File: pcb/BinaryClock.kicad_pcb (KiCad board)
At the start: 2 copper layers, 26.4 x 41.7 mm, 17 parts, among them CON1 AVR-ISP-6, IC1 ATMEGA328P-A, U1 MC33269, U3 clock_header, U4 clock_header, U5 clock_header, Y1 16MHz

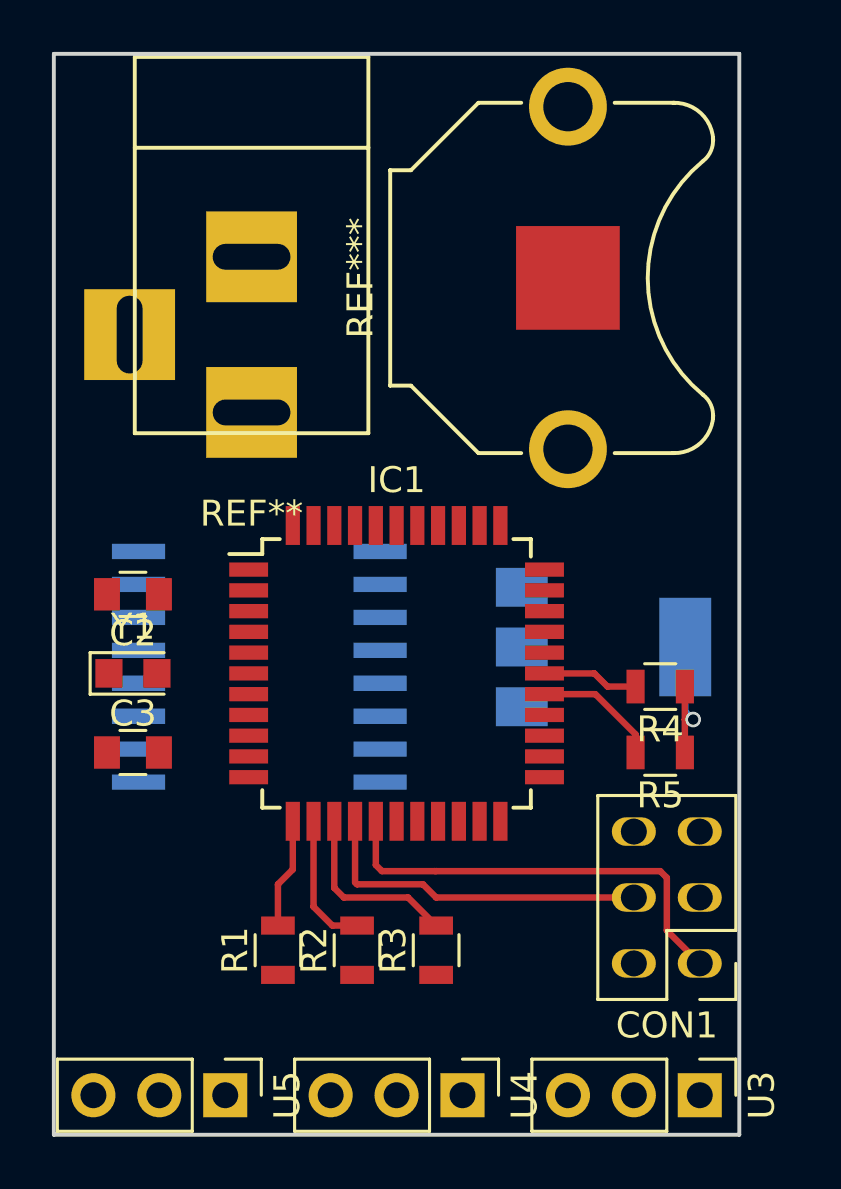
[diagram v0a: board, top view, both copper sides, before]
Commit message: Finished initial attempt at routing
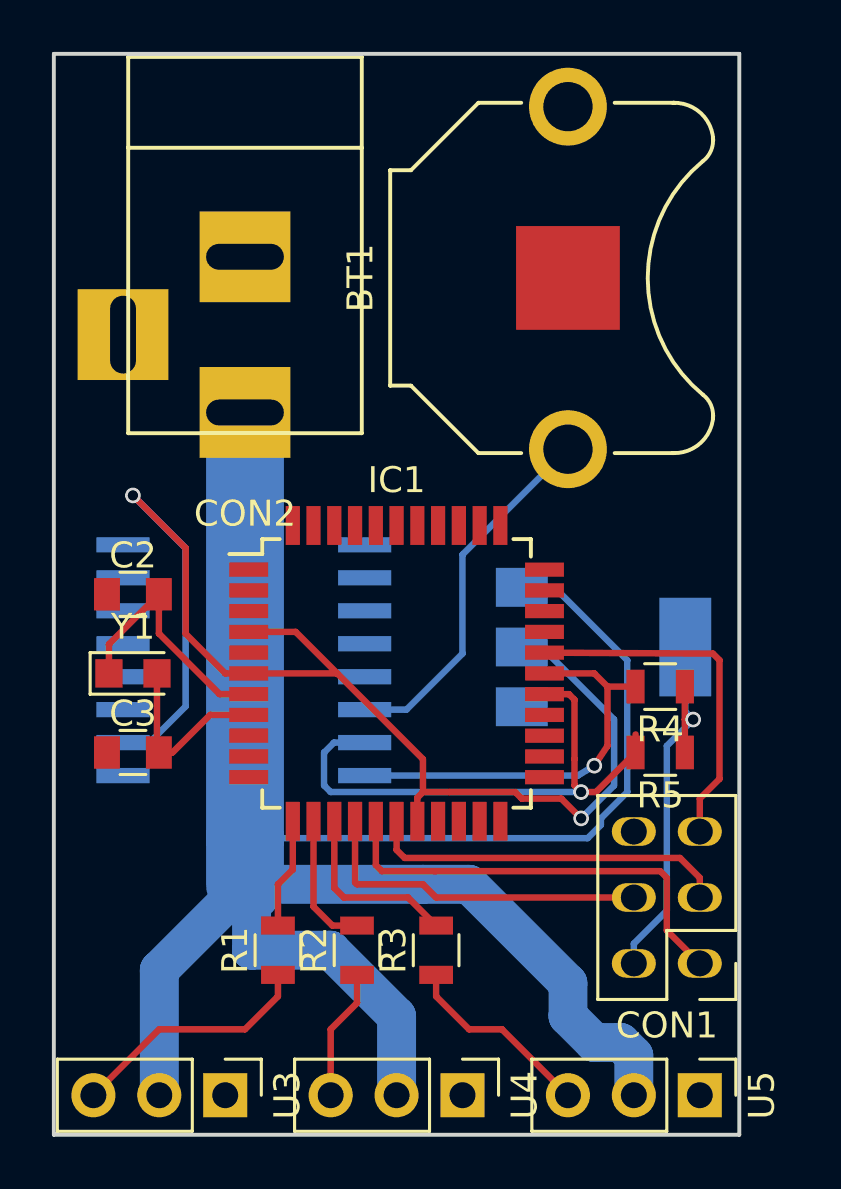
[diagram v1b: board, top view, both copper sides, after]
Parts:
- removed ?: , tapMatrix_Shield:DS3231
- removed REF**: BARREL_JACK, Connectors:BARREL_JACK
- removed REF***: Keystone_3001_1x12mm-CoinCell, Battery_Holders:Keystone_3001_1x12mm-CoinCell
- added BT1: Battery_Cell, Battery_Holders:Keystone_3001_1x12mm-CoinCell, F.Cu at (165.6, 65.5)
- added CON2: BARREL_JACK, Connectors:BARREL_JACK, F.Cu at (153.2, 64.5)
- added U2: DS3231, tapMatrix_Shield:DS3231, B.Cu at (153.4, 80.5)
- moved U3 18.3 mm to (152.4, 97.0)
- moved U5 18.3 mm to (170.7, 97.0)
- turned C2 to 0 degrees
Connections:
- IC1 pad 18: Net-(IC1-Pad18) -> VCC
- U3 pad 1: (no net) -> GND
- U3 pad 2: (no net) -> /VIN
- U3 pad 3: (no net) -> /LED1
- U4 pad 1: (no net) -> GND
- U4 pad 2: (no net) -> /VIN
- U4 pad 3: (no net) -> /LED2
- U5 pad 1: (no net) -> GND
- U5 pad 2: (no net) -> /VIN
- U5 pad 3: (no net) -> /LED3
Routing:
- net /VIN: track 0.00 -> 87.9 mm
- net VCC: track 5.78 -> 67.5 mm, vias 1 -> 3
- net SDA: track 4.85 -> 21.3 mm, vias 0 -> 1
- net Net-(BT1-Pad1): track 0.00 -> 14.2 mm
- net /SCK: track 0.00 -> 14.0 mm
- net /RESET: track 0.00 -> 13.8 mm
- net SCL: track 3.72 -> 15.9 mm, vias 0 -> 1
- net Net-(C2-Pad2): track 0.00 -> 9.78 mm
- net /LED1: track 0.00 -> 9.52 mm
- net /LED3: track 0.00 -> 7.49 mm
- net Net-(C3-Pad2): track 0.00 -> 7.14 mm
- net /LED2: track 0.00 -> 5.06 mm
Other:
- net class wide added: clearance 0.2, trace_width 3, via_dia 0.6, via_drill 0.4
